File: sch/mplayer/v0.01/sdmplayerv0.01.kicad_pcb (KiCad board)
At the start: 2 copper layers, 47.2 x 69.6 mm, 66 parts, among them CON1 SD_Card, IC1 AT24CS64-SSHM, P1 USB_OTG, P2 CONN_01X09, P3 ClockBat, P4 USART1, P5 AudioJack, P6 LiPo battery, SW1 SW_PUSH, U1 VS1053, U2 LM3671MF-3.3, U3 STM32F103RCTx, U4 BQ24090, U5 BQ27510, U6 NCP1117ST18T3G, Y1 12.288MHz, Y2 8MHz, Y3 32768Hz

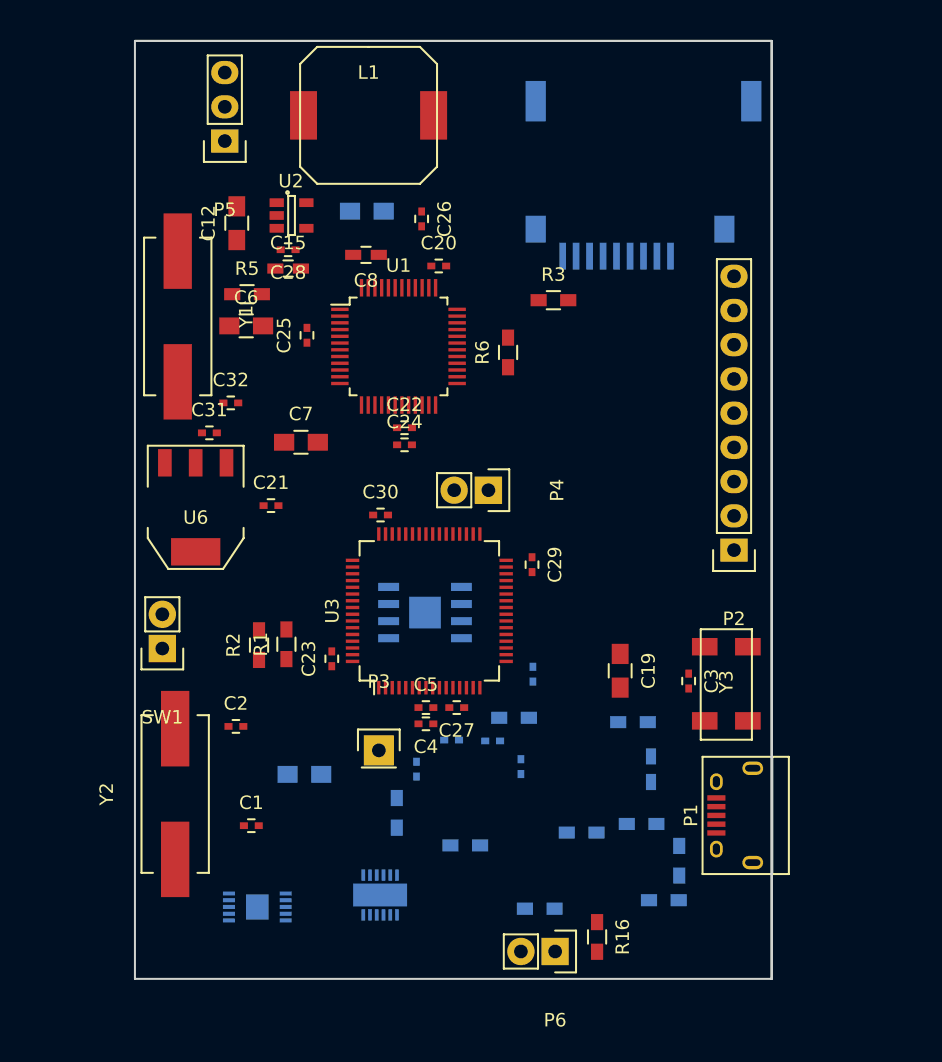
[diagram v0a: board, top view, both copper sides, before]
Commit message: upd
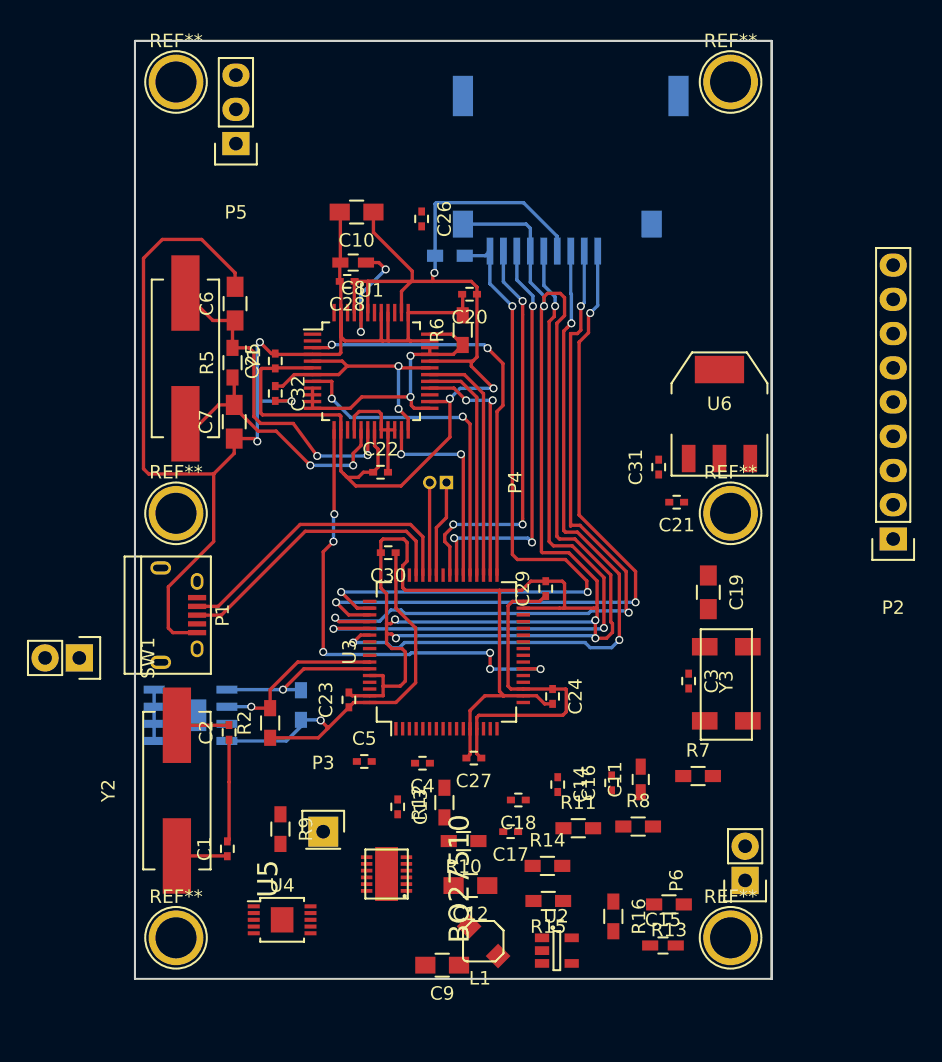
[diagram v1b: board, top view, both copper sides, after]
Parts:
- added REF**: 1pin, Connect:1pin, F.Cu at (188.0, 124.5)
- added REF**: 1pin, Connect:1pin, F.Cu at (188.0, 92.5)
- added REF**: 1pin, Connect:1pin, F.Cu at (188.0, 156.0)
- added REF**: 1pin, Connect:1pin, F.Cu at (146.8, 156.0)
- added REF**: 1pin, Connect:1pin, F.Cu at (146.8, 124.5)
- added REF**: 1pin, Connect:1pin, F.Cu at (146.8, 92.5)
- C10, C11, C13, C14, C16, C17, C18, C9, R10, R11, R12, R13, R14, R15, R7, R8, R9, U4, U5: moved to F.Cu
- L1: footprint Inductors:self_cms_we-tpc_XL -> v0:CDRH2D14
- R1, R3: moved to B.Cu
- moved L1 61.9 mm to (169.6, 156.2)
- moved U2 58.0 mm to (175.1, 156.9)
- moved C15 57.4 mm to (182.9, 156.5)
- moved C12 52.1 mm to (168.7, 152.1), turned to 180 degrees
- moved P1 44.2 mm to (146.8, 132.0), turned to 270 degrees
- moved U6 39.5 mm to (187.1, 117.1), turned to 0 degrees
- moved C31 33.4 mm to (182.6, 121.0), turned to 90 degrees
- moved C21 30.1 mm to (184.0, 123.6), turned to 180 degrees
- moved C24 21.7 mm to (174.8, 138.0), turned to 270 degrees
- moved IC1 19.0 mm to (147.9, 139.4), turned to 0 degrees
- moved R12 18.0 mm to (166.7, 145.9), turned to 90 degrees
- moved C9 17.5 mm to (166.6, 158.0)
- moved P6 15.1 mm to (189.0, 151.7), turned to 90 degrees
- moved P2 11.8 mm to (200.0, 126.4)
- moved R14 11.3 mm to (174.4, 150.6)
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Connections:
- C31 pad 2: Net-(C31-Pad2) -> GND
- C32 pad 2: Net-(C31-Pad2) -> GND
- U6 pad 1: Net-(C31-Pad2) -> GND
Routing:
- net GND: track 0.00 -> 283.6 mm, vias 0 -> 8
- net +3V3: track 0.00 -> 149.6 mm, vias 0 -> 4
- net /DAT3: track 0.00 -> 55.1 mm, vias 0 -> 3
- net /SD_CLK: track 0.00 -> 53.8 mm, vias 0 -> 3
- net /SD_CONN: track 0.00 -> 53.7 mm, vias 0 -> 3
- net /DAT2: track 0.00 -> 53.5 mm, vias 0 -> 3
- net /SD_CMD: track 0.00 -> 53.3 mm, vias 0 -> 3
- net /xDCS: track 0.00 -> 35.6 mm, vias 0 -> 6
- net /DAT0: track 0.00 -> 30.9 mm, vias 0 -> 3
- net /xRST: track 0.00 -> 30.7 mm, vias 0 -> 2
- net /DAT1: track 0.00 -> 30.2 mm, vias 0 -> 3
- net /DREQ: track 0.00 -> 25.0 mm, vias 0 -> 2
- net Net-(C6-Pad1): track 0.00 -> 24.9 mm, vias 0 -> 2
- net /USB_DM: track 0.00 -> 22.5 mm
- net Net-(R6-Pad1): track 0.00 -> 21.8 mm, vias 0 -> 2
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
